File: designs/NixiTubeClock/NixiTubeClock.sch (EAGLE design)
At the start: 15 parts, among them IC1 74141N, IC2 74HCT595D, IC3 74141N, IC4 74141N, IC5 74HCT595D, IC6 74141N

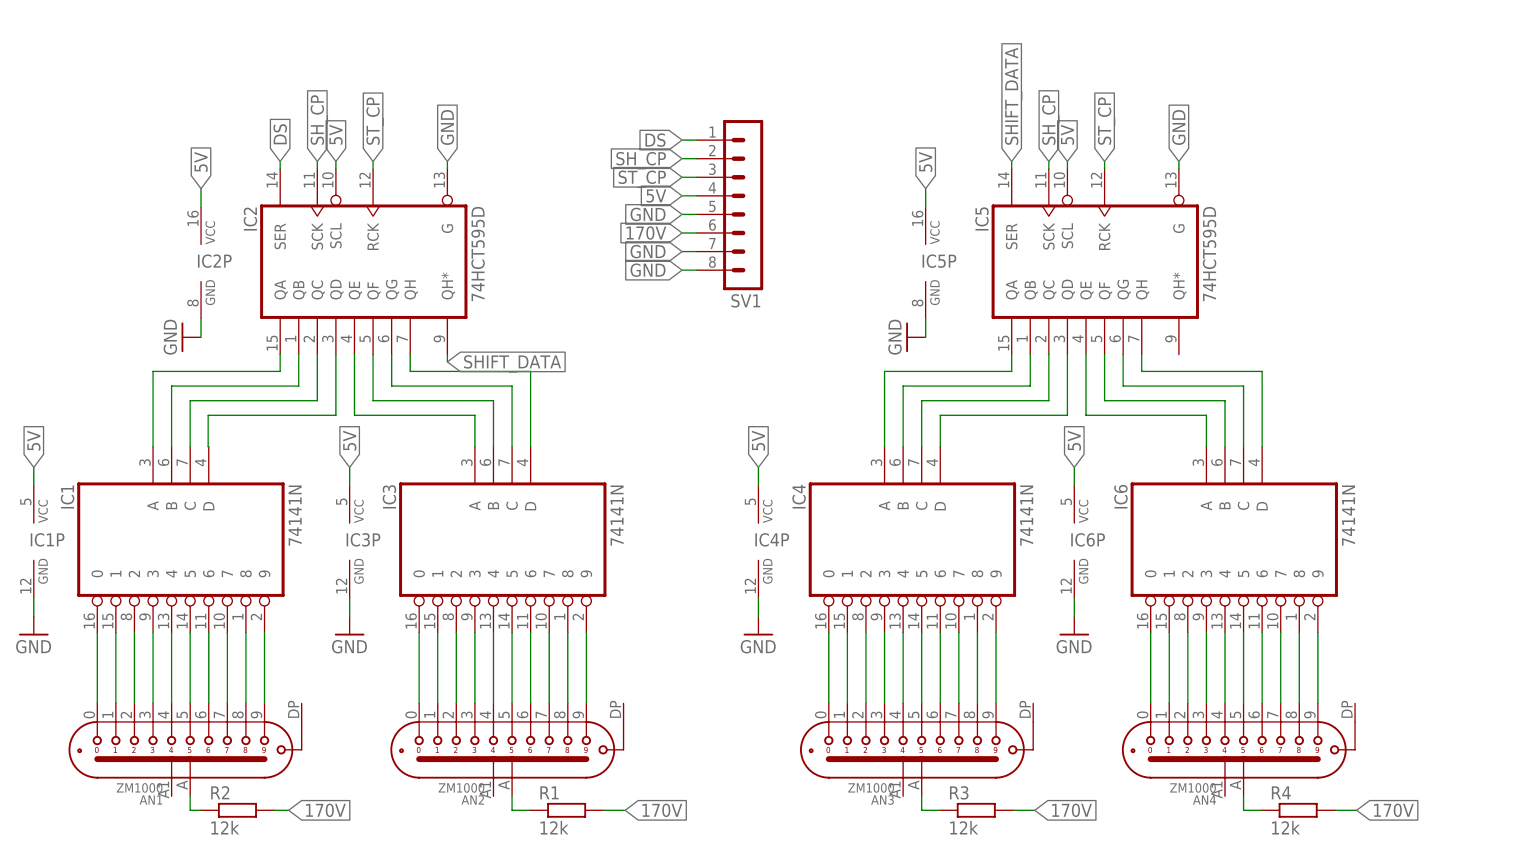
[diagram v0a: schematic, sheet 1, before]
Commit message: added new nixi clock design top board
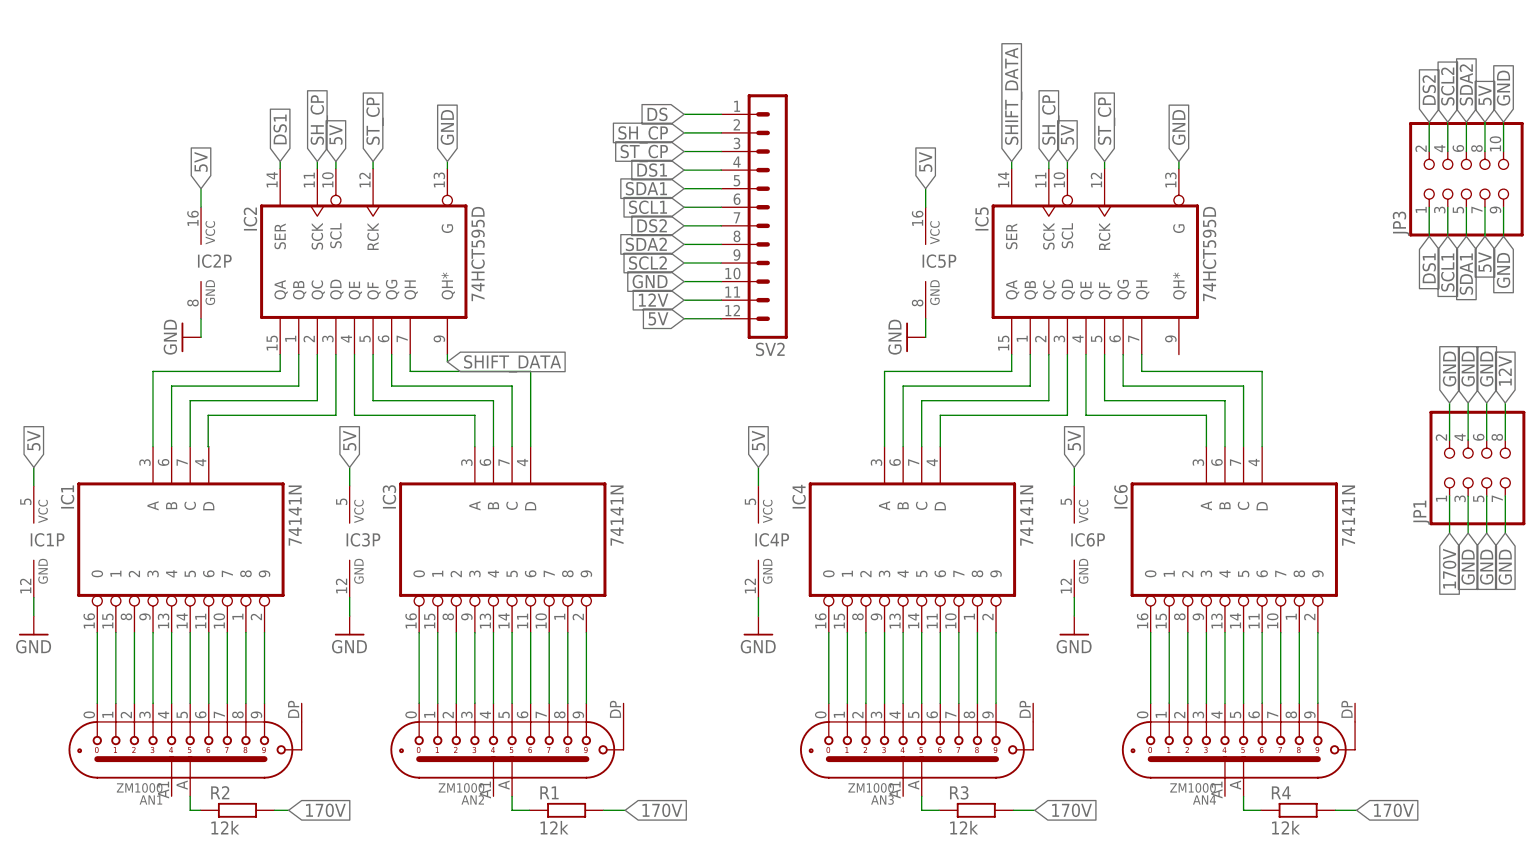
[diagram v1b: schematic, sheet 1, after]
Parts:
- removed SV1: (no value), con-lstb:MA08-1
- added JP1: (no value), pinhead:PINHD-2X4/90
- added JP3: (no value), pinhead:PINHD-2X5/90
- added SV2: (no value), con-lstb:MA12-1
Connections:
- new net 12V: JP1.8, SV2.11
- new net DS1: IC2A.SER, JP3.1, SV2.4
- new net DS2: JP3.2, SV2.7
- new net SCL1: JP3.3, SV2.6
- new net SCL2: JP3.4, SV2.9
- new net SDA1: JP3.5, SV2.5
- new net SDA2: JP3.6, SV2.8
- net 170V: now also JP1.1; no longer SV1.6
- net 5V: now also JP3.7, JP3.8, SV2.12; no longer SV1.4
- net DS: now also SV2.1; no longer IC2A.SER, SV1.1
- net GND: now also JP1.2, JP1.3, JP1.4, JP1.5, JP1.6, JP1.7, JP3.10, JP3.9, SV2.10; no longer SV1.5, SV1.7, SV1.8
- net SH_CP: now also SV2.2; no longer SV1.2
- net ST_CP: now also SV2.3; no longer SV1.3
